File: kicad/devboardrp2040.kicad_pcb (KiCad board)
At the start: 2 copper layers, 31.5 x 25.5 mm, 41 parts, among them J1 Conn_01x12_Pin, J2 Conn_01x12_Pin, SW1 SW_Push, SW2 SW_Push, U1 AP63203WU-7, U2 GT-USB-7010ASV, U4 W25Q64JVSSIQ_C179171, U5 ABM8-272-T3_C20625731, U6 RP2350A-QFN60

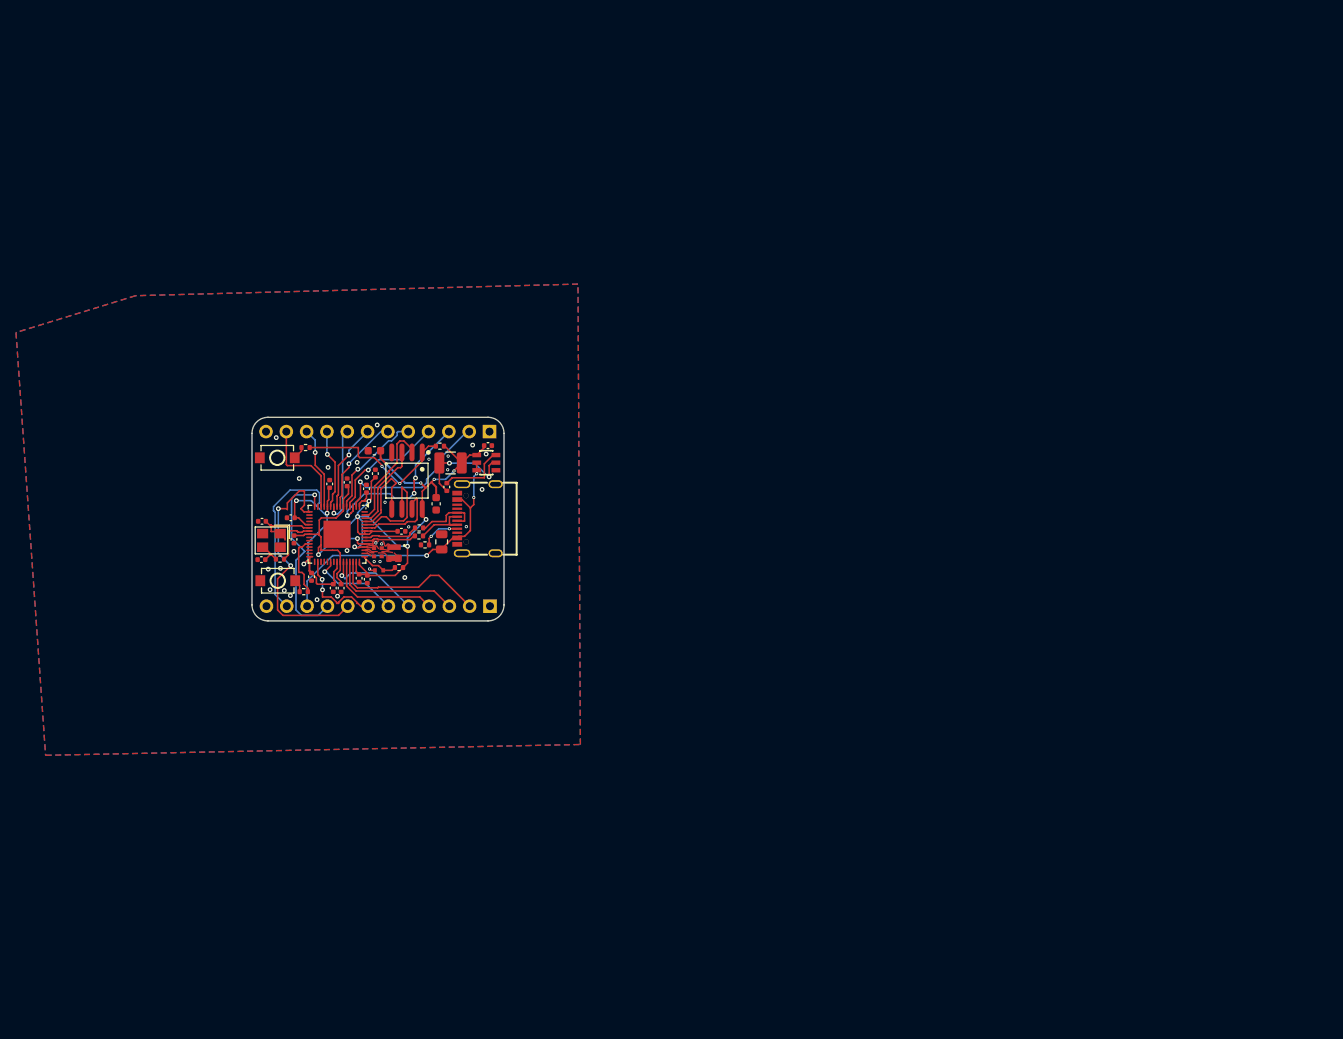
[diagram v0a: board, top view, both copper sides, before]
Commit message: hiii
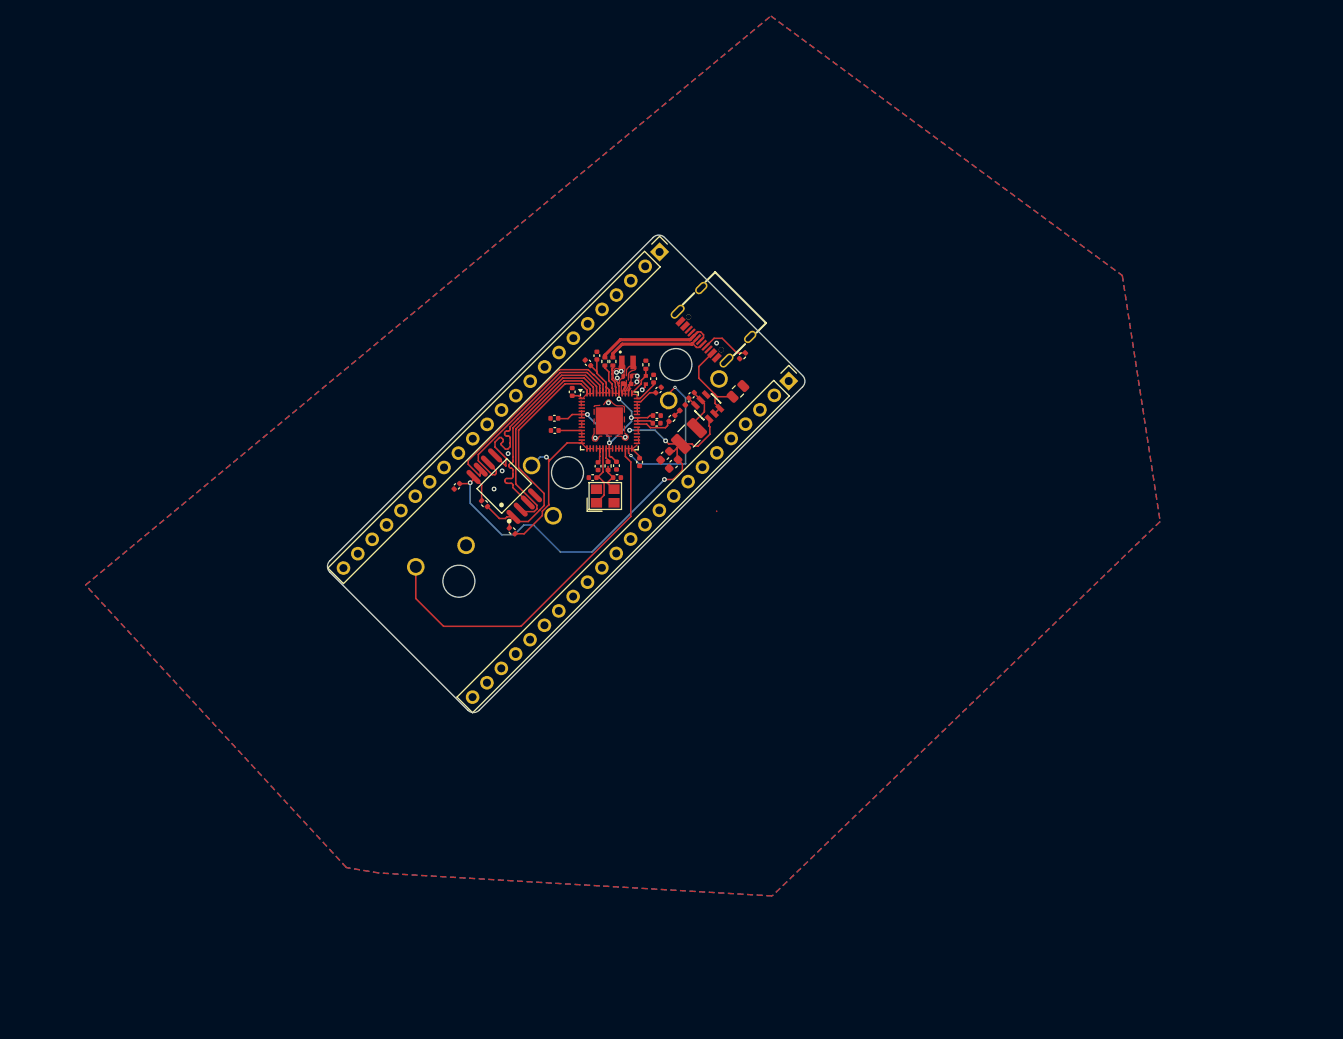
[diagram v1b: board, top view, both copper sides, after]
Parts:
- removed R8: 1k, Resistor_SMD:R_0402_1005Metric
- removed SW2: SW_Push, easyeda2kicad:SW-SMD_L3.9-W3.0-P4.45
- added D1: LED, LED_SMD:LED_0402_1005Metric, F.Cu at (102.6, 28.6)
- added R9: 33, Resistor_SMD:R_0402_1005Metric, F.Cu at (101.2, 29.9)
- added SW3: SW_Push, Button_Switch_Keyboard:SW_Cherry_MX_1.00u_Plate, B.Cu at (69.2, 48.4)
- added SW4: SW_Push, Button_Switch_Keyboard:SW_Cherry_MX_1.00u_Plate, B.Cu at (107.1, 25.0)
- J1, J2: value Conn_01x12_Pin -> Conn_01x23_Pin; footprint Connector_PinHeader_2.54mm:PinHeader_1x12_P2.54mm_Vertical -> Connector_PinHeader_2.54mm:PinHeader_1x23_P2.54mm_Vertical; moved to F.Cu
- SW1: footprint easyeda2kicad:SW-SMD_L3.9-W3.0-P4.45 -> Button_Switch_Keyboard:SW_Cherry_MX_1.00u_Plate; moved to B.Cu
- moved J2 46.8 mm to (115.8, 25.2), turned to -45 degrees
- moved R1 46.2 mm to (110.1, 22.1), turned to 45 degrees
- moved C24 45.6 mm to (94.4, 37.3), turned to 180 degrees
- moved C10 45.0 mm to (99.4, 29.5), turned to 0 degrees
- moved C14 43.4 mm to (99.6, 26.3), turned to 45 degrees
- moved R5 42.6 mm to (93.3, 35.8), turned to 90 degrees
- moved C17 42.6 mm to (99.0, 24.9)
- moved U5 42.1 mm to (92.9, 39.6), turned to 0 degrees
- moved C23 41.7 mm to (91.3, 37.3)
- moved C1 41.5 mm to (109.5, 26.5), turned to 45 degrees
- moved C18 41.4 mm to (97.2, 35.4)
- moved C7 41.0 mm to (98.0, 25.1), turned to 90 degrees
- moved R2 39.9 mm to (98.0, 23.2), turned to -90 degrees
- moved C19 38.4 mm to (92.0, 35.9)
- moved U2 38.1 mm to (106.3, 18.3), turned to 135 degrees
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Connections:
- J1 pad 10: Net-(J1-Pin_10) -> unconnected-(J1-Pin_10-Pad10)
- J1 pad 11: Net-(J1-Pin_11) -> GND
- J1 pad 12: GND -> unconnected-(J1-Pin_12-Pad12)
- J1 pad 2: Net-(J1-Pin_2) -> unconnected-(J1-Pin_2-Pad2)
- J1 pad 3: Net-(J1-Pin_3) -> unconnected-(J1-Pin_3-Pad3)
- J1 pad 4: Net-(J1-Pin_4) -> unconnected-(J1-Pin_4-Pad4)
- J1 pad 5: Net-(J1-Pin_5) -> unconnected-(J1-Pin_5-Pad5)
- J1 pad 6: Net-(J1-Pin_6) -> GND
- J1 pad 7: Net-(J1-Pin_7) -> unconnected-(J1-Pin_7-Pad7)
- J1 pad 8: Net-(J1-Pin_8) -> unconnected-(J1-Pin_8-Pad8)
- J1 pad 9: Net-(J1-Pin_9) -> unconnected-(J1-Pin_9-Pad9)
- J2 pad 10: USB_VBUS -> unconnected-(J2-Pin_10-Pad10)
- J2 pad 11: +3V3 -> GND
- J2 pad 12: GND -> unconnected-(J2-Pin_12-Pad12)
- J2 pad 2: Net-(J2-Pin_2) -> unconnected-(J2-Pin_2-Pad2)
- J2 pad 3: Net-(J2-Pin_3) -> unconnected-(J2-Pin_3-Pad3)
- J2 pad 4: Net-(J2-Pin_4) -> unconnected-(J2-Pin_4-Pad4)
- J2 pad 5: Net-(J2-Pin_5) -> unconnected-(J2-Pin_5-Pad5)
- J2 pad 6: GPIO24 -> GND
- J2 pad 7: GPIO20 -> unconnected-(J2-Pin_7-Pad7)
- J2 pad 8: GPIO12 -> unconnected-(J2-Pin_8-Pad8)
- J2 pad 9: GPIO11 -> unconnected-(J2-Pin_9-Pad9)
- R4 pad 2: Net-(R4-Pad2) -> GPIO11
- SW1 pad 2: Net-(R4-Pad2) -> GPIO11
- U6 pad 10: Net-(J1-Pin_9) -> unconnected-(U6-GPIO7-Pad10)
- U6 pad 12: Net-(J1-Pin_10) -> unconnected-(U6-GPIO8-Pad12)
- U6 pad 13: Net-(J1-Pin_11) -> unconnected-(U6-GPIO9-Pad13)
- U6 pad 2: Net-(J1-Pin_2) -> unconnected-(U6-GPIO0-Pad2)
- U6 pad 28: unconnected-(U6-GPIO17-Pad28) -> Net-(U6-GPIO17)
- U6 pad 29: unconnected-(U6-GPIO18-Pad29) -> Net-(U6-GPIO18)
- U6 pad 3: Net-(J1-Pin_3) -> unconnected-(U6-GPIO1-Pad3)
- U6 pad 37: unconnected-(U6-GPIO25-Pad37) -> Net-(U6-GPIO25)
- U6 pad 4: Net-(J1-Pin_4) -> unconnected-(U6-GPIO2-Pad4)
- U6 pad 40: Net-(J2-Pin_5) -> unconnected-(U6-GPIO26_ADC0-Pad40)
- U6 pad 41: Net-(J2-Pin_4) -> unconnected-(U6-GPIO27_ADC1-Pad41)
- U6 pad 42: Net-(J2-Pin_3) -> unconnected-(U6-GPIO28_ADC2-Pad42)
- U6 pad 43: Net-(J2-Pin_2) -> unconnected-(U6-GPIO29_ADC3-Pad43)
- U6 pad 5: Net-(J1-Pin_5) -> unconnected-(U6-GPIO3-Pad5)
- U6 pad 60: unconnected-(U6-QSPI_SS-Pad60) -> Net-(U4-~{CS})
- U6 pad 7: Net-(J1-Pin_6) -> unconnected-(U6-GPIO4-Pad7)
- U6 pad 8: Net-(J1-Pin_7) -> unconnected-(U6-GPIO5-Pad8)
- U6 pad 9: Net-(J1-Pin_8) -> unconnected-(U6-GPIO6-Pad9)
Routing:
- net +3V3: track 132.1 -> 85.3 mm, vias 12 -> 4
- net Net-(U6-GPIO17): track 0.00 -> 46.7 mm
- net GPIO12: track 32.1 -> 0.00 mm, vias 2 -> 0
- net USB_VBUS: track 37.3 -> 11.9 mm, vias 3 -> 0
- net Net-(U6-GPIO18): track 0.00 -> 22.1 mm, vias 0 -> 2
- net Net-(J1-Pin_3): track 21.3 -> 0.00 mm, vias 3 -> 0
- net Net-(J1-Pin_2): track 20.9 -> 0.00 mm, vias 1 -> 0
- net Net-(J2-Pin_2): track 20.1 -> 0.00 mm
- net Net-(J2-Pin_3): track 16.4 -> 0.00 mm
- net IO0: track 11.6 -> 27.8 mm
- net IO3: track 11.3 -> 27.0 mm
- net Net-(J1-Pin_4): track 15.4 -> 0.00 mm, vias 1 -> 0
- net IO2: track 10.8 -> 26.0 mm
- net Net-(J2-Pin_4): track 14.4 -> 0.00 mm
- net Net-(J1-Pin_5): track 13.7 -> 0.00 mm, vias 1 -> 0
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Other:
- board size 31.5 x 25.5 mm -> 59.7 x 59.7 mm

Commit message: FINISHED KAUHdiodu
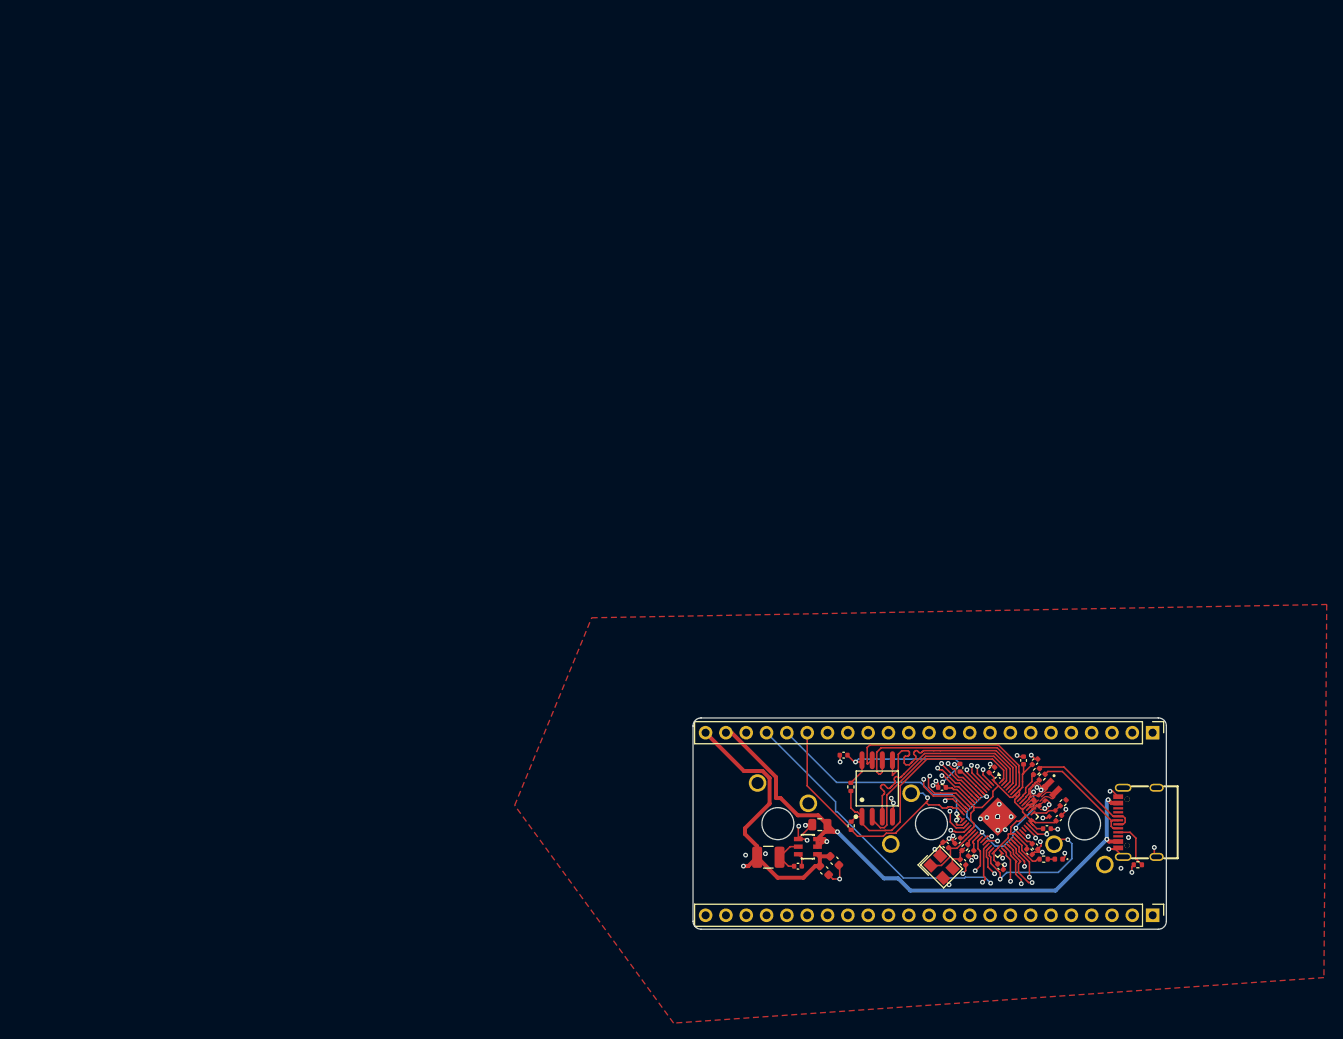
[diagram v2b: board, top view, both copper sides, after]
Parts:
- L1: value 47uh -> 3.9uh
- moved J1 86.1 mm to (161.3, 69.2), turned to -90 degrees
- moved U2 81.7 mm to (159.4, 80.4), turned to 90 degrees
- moved J2 80.8 mm to (161.3, 92.0), turned to -90 degrees
- moved R1 80.6 mm to (159.5, 85.7), turned to 0 degrees
- moved SW4 77.5 mm to (155.4, 85.7), turned to 0 degrees
- moved R2 75.6 mm to (150.1, 77.9), turned to -135 degrees
- moved L2 75.1 mm to (148.7, 76.1), turned to -45 degrees
- moved C17 74.7 mm to (149.6, 79.8), turned to 45 degrees
- moved R6 74.7 mm to (147.5, 74.7), turned to -135 degrees
- moved C16 74.7 mm to (146.6, 72.8), turned to 45 degrees
- moved R7 74.4 mm to (146.8, 74.0), turned to 45 degrees
- moved C7 74.3 mm to (148.8, 79.3), turned to 45 degrees
- moved C5 73.9 mm to (147.5, 77.3), turned to -45 degrees
- moved C22 73.7 mm to (145.2, 72.6), turned to 90 degrees
- moved D1 73.4 mm to (149.6, 85.0), turned to 180 degrees
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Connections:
- J1 pad 10: unconnected-(J1-Pin_10-Pad10) -> GPIO5
- J1 pad 12: unconnected-(J1-Pin_12-Pad12) -> GPIO6
- J1 pad 13: unconnected-(J1-Pin_13-Pad13) -> GPIO7
- J1 pad 14: unconnected-(J1-Pin_14-Pad14) -> GPIO8
- J1 pad 15: unconnected-(J1-Pin_15-Pad15) -> GPIO9
- J1 pad 17: unconnected-(J1-Pin_17-Pad17) -> GPIO10
- J1 pad 18: unconnected-(J1-Pin_18-Pad18) -> GPIO11
- J1 pad 19: unconnected-(J1-Pin_19-Pad19) -> GPIO12
- J1 pad 2: unconnected-(J1-Pin_2-Pad2) -> +1V1
- J1 pad 20: unconnected-(J1-Pin_20-Pad20) -> RUN
- J1 pad 22: unconnected-(J1-Pin_22-Pad22) -> USB_VBUS
- J1 pad 23: unconnected-(J1-Pin_23-Pad23) -> +3V3
- J1 pad 3: unconnected-(J1-Pin_3-Pad3) -> GND
- J1 pad 4: unconnected-(J1-Pin_4-Pad4) -> GPIO0
- J1 pad 5: unconnected-(J1-Pin_5-Pad5) -> GPIO1
- J1 pad 7: unconnected-(J1-Pin_7-Pad7) -> GPIO2
- J1 pad 8: unconnected-(J1-Pin_8-Pad8) -> GPIO3
- J1 pad 9: unconnected-(J1-Pin_9-Pad9) -> GPIO4
- J2 pad 10: unconnected-(J2-Pin_10-Pad10) -> GPIO21
- J2 pad 12: unconnected-(J2-Pin_12-Pad12) -> GPIO19
- J2 pad 13: unconnected-(J2-Pin_13-Pad13) -> GPIO20
- J2 pad 14: unconnected-(J2-Pin_14-Pad14) -> GPIO16
- J2 pad 15: unconnected-(J2-Pin_15-Pad15) -> SWDIO
- J2 pad 17: unconnected-(J2-Pin_17-Pad17) -> SWCLK
- J2 pad 18: unconnected-(J2-Pin_18-Pad18) -> GPIO15
- J2 pad 19: unconnected-(J2-Pin_19-Pad19) -> GPIO14
- J2 pad 2: unconnected-(J2-Pin_2-Pad2) -> GPIO29
- J2 pad 20: unconnected-(J2-Pin_20-Pad20) -> GPIO13
- J2 pad 22: unconnected-(J2-Pin_22-Pad22) -> USB_VBUS
- J2 pad 23: unconnected-(J2-Pin_23-Pad23) -> +3V3
- J2 pad 3: unconnected-(J2-Pin_3-Pad3) -> GPIO28
- J2 pad 4: unconnected-(J2-Pin_4-Pad4) -> GND
- J2 pad 5: unconnected-(J2-Pin_5-Pad5) -> GPIO26
- J2 pad 7: unconnected-(J2-Pin_7-Pad7) -> GPIO24
- J2 pad 8: unconnected-(J2-Pin_8-Pad8) -> GPIO23
- J2 pad 9: unconnected-(J2-Pin_9-Pad9) -> GPIO22
- U6 pad 10: unconnected-(U6-GPIO7-Pad10) -> GPIO7
- U6 pad 12: unconnected-(U6-GPIO8-Pad12) -> GPIO8
- U6 pad 13: unconnected-(U6-GPIO9-Pad13) -> GPIO9
- U6 pad 14: unconnected-(U6-GPIO10-Pad14) -> GPIO10
- U6 pad 17: unconnected-(U6-GPIO13-Pad17) -> GPIO13
- U6 pad 18: unconnected-(U6-GPIO14-Pad18) -> GPIO14
- U6 pad 19: unconnected-(U6-GPIO15-Pad19) -> GPIO15
- U6 pad 2: unconnected-(U6-GPIO0-Pad2) -> GPIO0
- U6 pad 24: unconnected-(U6-SWCLK-Pad24) -> SWCLK
- U6 pad 25: unconnected-(U6-SWDIO-Pad25) -> SWDIO
- U6 pad 27: unconnected-(U6-GPIO16-Pad27) -> GPIO16
- U6 pad 3: unconnected-(U6-GPIO1-Pad3) -> GPIO1
- U6 pad 31: unconnected-(U6-GPIO19-Pad31) -> GPIO19
- U6 pad 33: unconnected-(U6-GPIO21-Pad33) -> GPIO21
- U6 pad 34: unconnected-(U6-GPIO22-Pad34) -> GPIO22
- U6 pad 35: unconnected-(U6-GPIO23-Pad35) -> GPIO23
- U6 pad 4: unconnected-(U6-GPIO2-Pad4) -> GPIO2
- U6 pad 40: unconnected-(U6-GPIO26_ADC0-Pad40) -> GPIO26
- U6 pad 41: unconnected-(U6-GPIO27_ADC1-Pad41) -> GPIO27
- U6 pad 42: unconnected-(U6-GPIO28_ADC2-Pad42) -> GPIO28
- U6 pad 43: unconnected-(U6-GPIO29_ADC3-Pad43) -> GPIO29
- U6 pad 5: unconnected-(U6-GPIO3-Pad5) -> GPIO3
- U6 pad 7: unconnected-(U6-GPIO4-Pad7) -> GPIO4
- U6 pad 8: unconnected-(U6-GPIO5-Pad8) -> GPIO5
- U6 pad 9: unconnected-(U6-GPIO6-Pad9) -> GPIO6
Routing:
- net USB_VBUS: track 11.9 -> 90.9 mm, vias 0 -> 4
- net GND: track 0.85 -> 49.2 mm, vias 10 -> 50
- net RUN: track 0.00 -> 44.0 mm, vias 0 -> 2
- net GPIO13: track 0.00 -> 34.5 mm, vias 0 -> 1
- net +3V3: track 85.3 -> 118.7 mm, vias 4 -> 3
- net GPIO14: track 0.00 -> 30.3 mm, vias 0 -> 1
- net Net-(U6-GPIO17): track 46.7 -> 76.5 mm, vias 0 -> 1
- net GPIO15: track 0.00 -> 28.3 mm, vias 0 -> 1
- net GPIO29: track 0.00 -> 27.9 mm, vias 0 -> 1
- net GPIO12: track 0.00 -> 27.6 mm, vias 0 -> 1
- net SWCLK: track 0.00 -> 26.6 mm, vias 0 -> 1
- net GPIO26: track 0.00 -> 23.1 mm, vias 0 -> 1
- net SWDIO: track 0.00 -> 22.4 mm, vias 0 -> 1
- net GPIO10: track 0.00 -> 21.4 mm, vias 0 -> 1
- net +1V1: track 23.9 -> 44.8 mm, vias 7 -> 6
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- added copper zone on In1.Cu, net GND
- removed copper zone on B.Cu, net GND
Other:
- board size 59.7 x 59.7 mm -> 59.2 x 26.4 mm
- copper layers 2 -> 4
